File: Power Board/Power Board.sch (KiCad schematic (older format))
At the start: 55 parts, among them J1 Conn_02x10_Odd_Even, J2 Conn_01x02, J3 Conn_01x02, J4 Conn_01x02, J5 Conn_01x02, Q1 SI7135DP, Q2 SI7135DP, Q3 SI7135DP, Q4 SI7135DP, Q5 SI7135DP, Q6 SI7135DP, U1 LTC4417CGN, U2 TPS54308DDC, U3 LTC3130-1

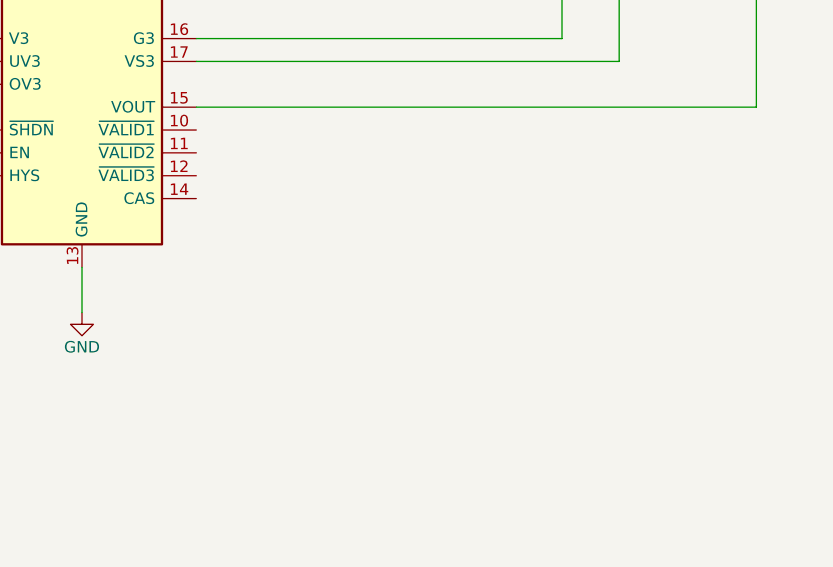
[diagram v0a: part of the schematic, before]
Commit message: a
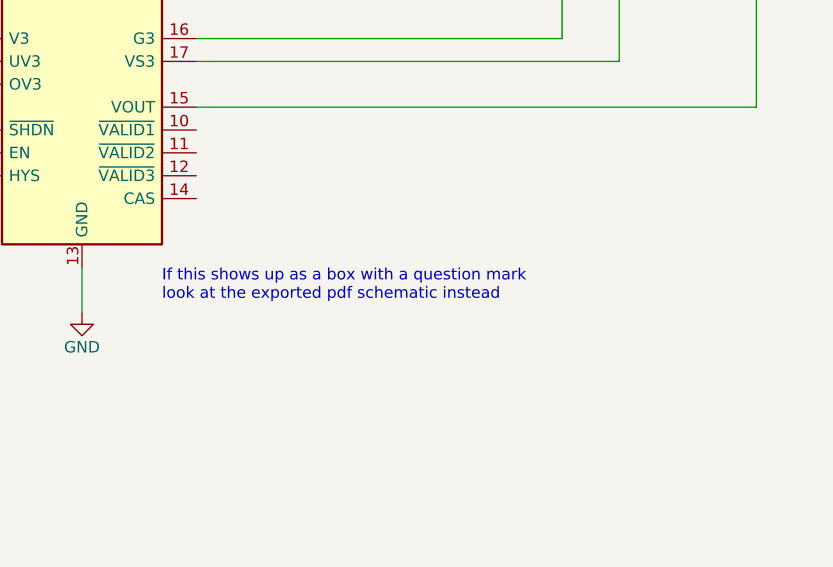
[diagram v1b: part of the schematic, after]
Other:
- note added: "If this shows up as a box with a question mark\nlook at the exported pdf schematic instead"
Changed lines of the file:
@@
 encoding utf-8
 Sheet 1 1
-Title ""
-Date ""
-Rev ""
-Comp ""
+Title "Avionics Power Board"
+Date "2018-03-20"
+Rev "0.8"
+Comp "UAH SHC Spaceport America Cup"
 Comment1 ""
 Comment2 ""
@@
 Text Notes 4050 600  0    50   ~ 0
 Power Supply Selector
+Text Notes 4950 5050 0    50   ~ 0
+If this shows up as a box with a question mark\nlook at the exported pdf schematic instead
 $EndSCHEMATC
